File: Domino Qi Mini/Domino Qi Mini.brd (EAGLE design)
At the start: 55.9 x 33 mm, 97 parts, among them J1 MH22-1, J2 MH22-1, M1 DOMINO, Q1 AP2302GN, Q2 2SC4081, SW1 IT-1100, SW2 IT-1100, SW3 IT-1100, U1 ATMEGA32U4-XUMU, U2 MP2162GQH, U3 NTB0104GU12, U4 NTB0102GU, U5 MAX3375EEKA+T, Y1 16MHz

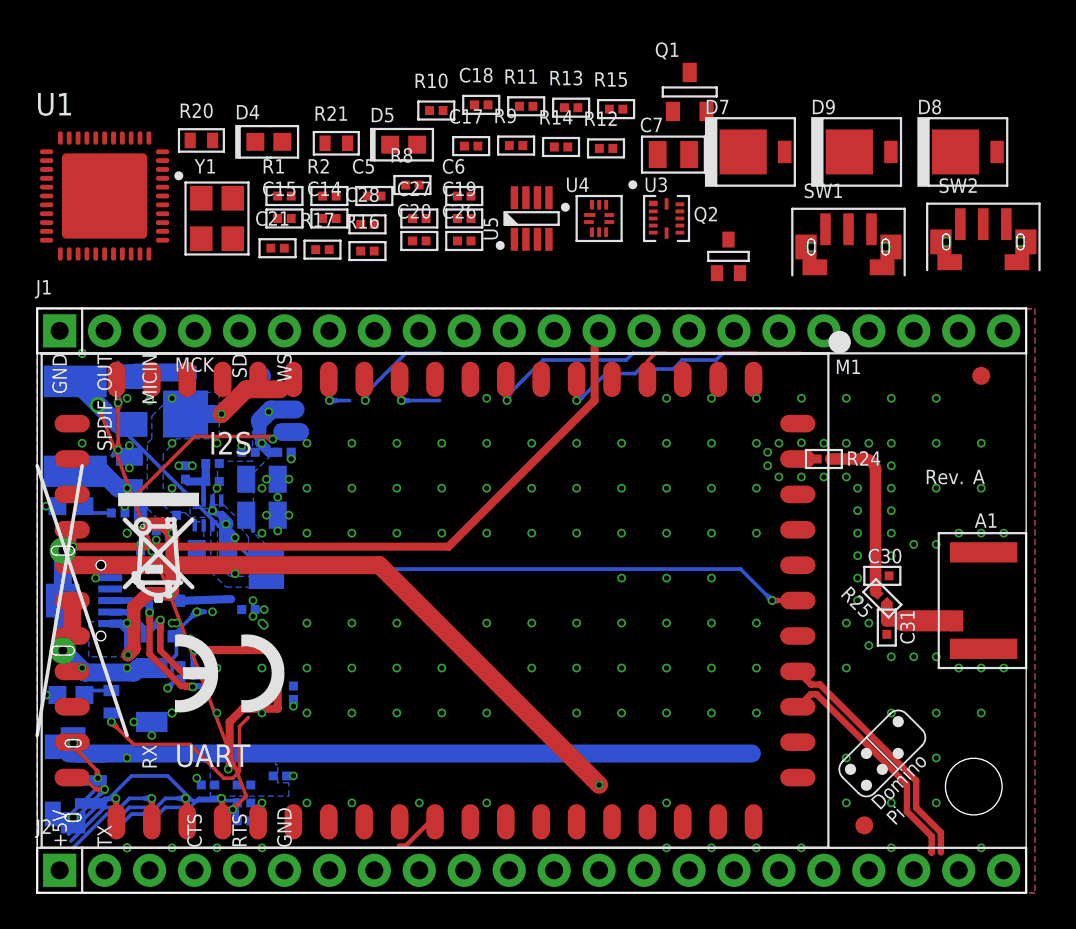
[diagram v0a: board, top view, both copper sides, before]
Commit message: Domino Qi Mini: work in progress
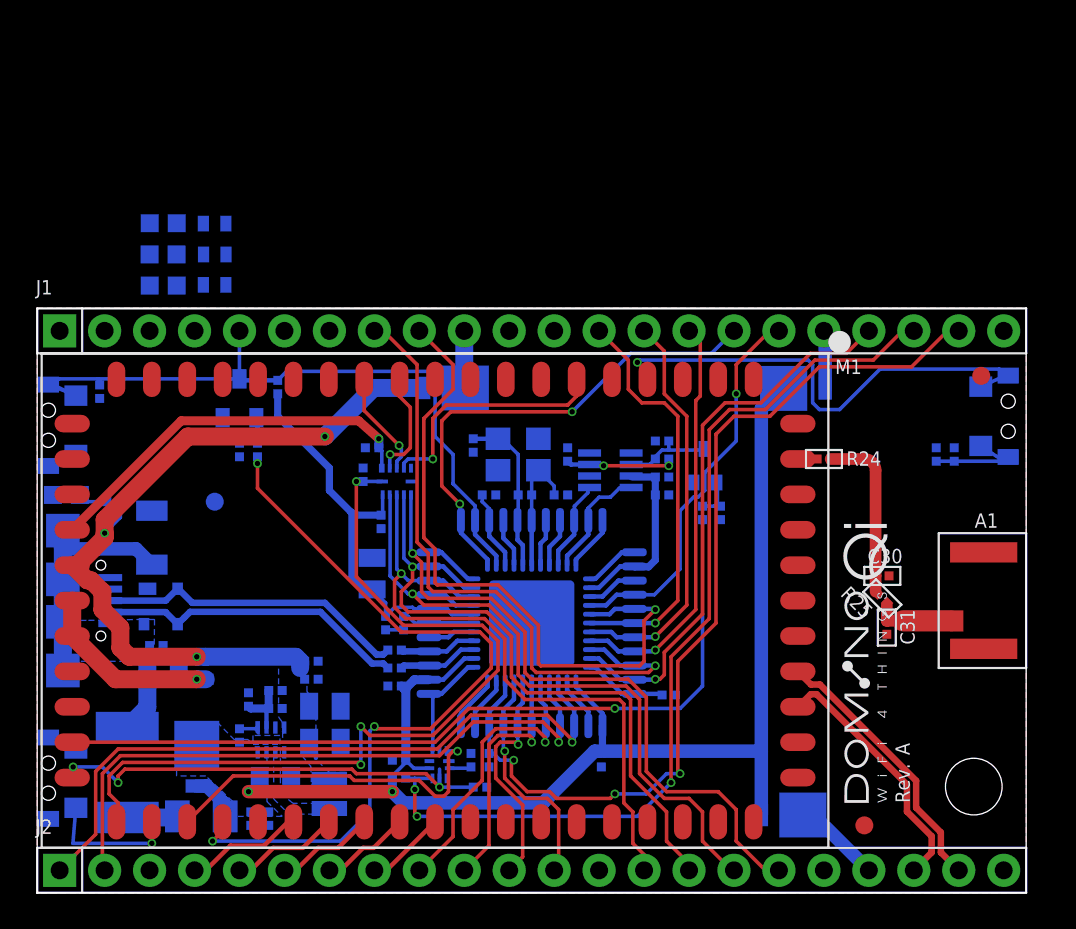
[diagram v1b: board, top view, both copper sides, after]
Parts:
- removed U$39: (no value), Domino:RECYCLE_BIN_LOGO
- removed U$41: (no value), Domino:CE_LOGO_SMALL
- removed U$9: (no value), Domino:DOMINO_LOGO_SMALL
- added U$3, U$5: (no value), Domino:DOMINO_QI_LOGO_SMALL
- S1: value USB_MR5-003A -> USB_MR5-001; device Domino:USB_MR5-003A -> Domino:USB-MR5-001
- SW1, SW2, SW3: value IT-1100 -> IT-1210; device Domino:IT-1100 -> Domino:IT-1210
- U$7: value (none) -> DOMINO_QI_LOGO; device Domino:DOMINO_LOGO_SMALL -> Domino:DOMINO_QI_LOGO
- U1: value ATMEGA32U4-XUMU -> ATMEGA32U4-XUAU/MU; device Domino:QFN44ML7X7 -> Domino:ATMEGA32U4_DUAL_FOOTPRINT
- moved U$7 98.7 mm to (-34.3, -47.0)
- moved SW2 60.9 mm to (0.64, 6.48), flipped to the bottom, turned to 270 degrees
- moved SW3 56.7 mm to (54.9, 26.9)
- moved SW1 46.3 mm to (0.64, 26.4), flipped to the bottom, turned to 270 degrees
- moved R23 45.2 mm to (51.8, 24.8), turned to 270 degrees
- moved C29 43.8 mm to (50.8, 24.8), turned to 90 degrees
- moved D9 37.9 mm to (41.6, 4.39), flipped to the bottom
- moved C14 34.2 mm to (31.9, 7.49), flipped to the bottom, turned to 270 degrees
- moved U1 34.1 mm to (27.9, 15.2), flipped to the bottom, turned to 180 degrees
- moved D8 33.8 mm to (22.5, 28.5), flipped to the bottom
- moved R8 33.5 mm to (20.4, 6.48), flipped to the bottom
- moved U4 32.2 mm to (22.7, 7.24), flipped to the bottom
- moved R17 31.6 mm to (25.0, 5.97), flipped to the bottom
- moved Q1 30.8 mm to (11.4, 27.9), flipped to the bottom
- moved C27 30.7 mm to (24.5, 7.49), flipped to the bottom, turned to 90 degrees
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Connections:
- net !RESET: now also SW1.1, U1.13A, U1.13M; no longer SW1.2, U1.13
- net +5V: now also U1.14A, U1.14M, U1.24A, U1.24M, U1.2A, U1.2M, U1.34A, U1.34M, U1.44A, U1.44M, U1.7A, U1.7M; no longer U1.14, U1.2, U1.24, U1.34, U1.44, U1.7
- net A0: now also U1.36A, U1.36M; no longer U1.36
- net A1: now also U1.37A, U1.37M; no longer U1.37
- net A2: now also U1.38A, U1.38M; no longer U1.38
- net A3: now also U1.39A, U1.39M; no longer U1.39
- net A4: now also U1.40A, U1.40M; no longer U1.40
- net A5: now also U1.41A, U1.41M; no longer U1.41
- net AREF: now also U1.42A, U1.42M; no longer U1.42
- net D+: now also D1.2; no longer D1.3
- net D-: now also D1.3; no longer D1.2
- net D4: now also U1.25A, U1.25M; no longer U1.25
- net D5: now also U1.31A, U1.31M; no longer U1.31
- net D6: now also U1.27A, U1.27M; no longer U1.27
- net GND: now also SW1.2, SW1.SH$1, SW1.SH$2, SW2.SH$1, SW2.SH$2, SW3.SH$1, SW3.SH$2, U1.15A, U1.15M, U1.23A, U1.23M, U1.35A, U1.35M, U1.43A, U1.43M, U1.5A, U1.5M, U1.PAD; no longer SW1.1, SW1.S$1, SW1.S$2, SW2.S$1, SW2.S$2, SW3.S$1, SW3.S$2, U1.15, U1.23, U1.35, U1.43, U1.5, U1.EXP
- net HANDSHAKE: now also U1.1A, U1.1M; no longer U1.1
- net IO10: now also U1.30A, U1.30M; no longer U1.30
- net IO11: now also U1.12A, U1.12M; no longer U1.12
- net IO12: now also U1.26M
- net IO13: now also U1.32A, U1.32M; no longer U1.32
- net IO8: now also U1.28A, U1.28M; no longer U1.28
- net IO9: now also U1.29A, U1.29M; no longer U1.29
- net MISO: now also U1.11A, U1.11M; no longer U1.11
- net MOSI: now also U1.10A, U1.10M; no longer U1.10
- net N$5: now also U1.3A, U1.3M; no longer U1.3
- net N$8: now also U1.33A, U1.33M; no longer U1.33
- net N$9: now also U1.4A, U1.4M; no longer U1.4
- net PE: now also S1.SH$1, S1.SH$2, S1.SH$3, S1.SH$4; no longer S1.S$1, S1.S$2, S1.S$3
- net RXD1: now also U1.20A, U1.20M; no longer U1.20
- net SCK: now also U1.9A, U1.9M; no longer U1.9
- net SCL: now also U1.18A, U1.18M; no longer U1.18
- net SDA: now also U1.19A, U1.19M; no longer U1.19
- net SS: now also U1.8A, U1.8M; no longer U1.8
- net TXD1: now also U1.21A, U1.21M; no longer U1.21
- net UCAP: now also U1.6A, U1.6M; no longer U1.6
- net XTAL1: now also U1.17A, U1.17M; no longer U1.17
- net XTAL2: now also U1.16A, U1.16M; no longer U1.16
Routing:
- net UART_RTS: track 75.6 -> 0.00 mm, vias 3 -> 0
- net GP6: track 0.00 -> 53.6 mm, vias 0 -> 3
- net AREF: track 0.00 -> 51.0 mm, vias 0 -> 3
- net +5V: track 46.5 -> 96.3 mm, vias 1 -> 2
- net I2S_MCK: track 7.10 -> 47.1 mm, vias 1 -> 3
- net MISO: track 0.00 -> 38.5 mm, vias 0 -> 1
- net SPDIF_OUT: track 8.13 -> 46.5 mm
- net !RESET: track 0.00 -> 37.7 mm
- net SS: track 0.00 -> 36.6 mm, vias 0 -> 1
- net A0: track 0.00 -> 36.4 mm, vias 0 -> 1
- net D6: track 0.00 -> 35.5 mm, vias 0 -> 1
- net MOSI: track 0.00 -> 35.2 mm, vias 0 -> 1
- net SCK: track 0.00 -> 34.8 mm, vias 0 -> 1
- net A1: track 0.00 -> 34.0 mm, vias 0 -> 1
- net D5: track 0.00 -> 33.6 mm, vias 0 -> 1
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- removed copper zone on layer 16, net +2V5
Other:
- board text removed: "CTS"
- board text removed: "Domino Core"
- board text removed: "Domino Pi"
- board text removed: "Domino Qi"
- board text removed: "MCK"
- board text removed: "MICIN"
- board text removed: "RTS"
- board text removed: "RX"
- board text removed: "SD"
- board text removed: "TX"
- board text removed: "WS"
